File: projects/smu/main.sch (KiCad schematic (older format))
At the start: 2 parts, among them P101 CONN_01X15, P102 CONN_01X34

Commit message: generate net and parts
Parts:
- P102: footprint (none) -> Pin_Headers:Pin_Header_Straight_1x34
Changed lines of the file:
@@
 F 0 "P102" H 5300 4400 50  0000 C CNN
 F 1 "CONN_01X34" V 5400 2650 50  0000 C CNN
-F 2 "" H 5300 2650 50  0000 C CNN
+F 2 "Pin_Headers:Pin_Header_Straight_1x34" H 5300 2650 50  0001 C CNN
 F 3 "" H 5300 2650 50  0000 C CNN
 	1    5300 2650

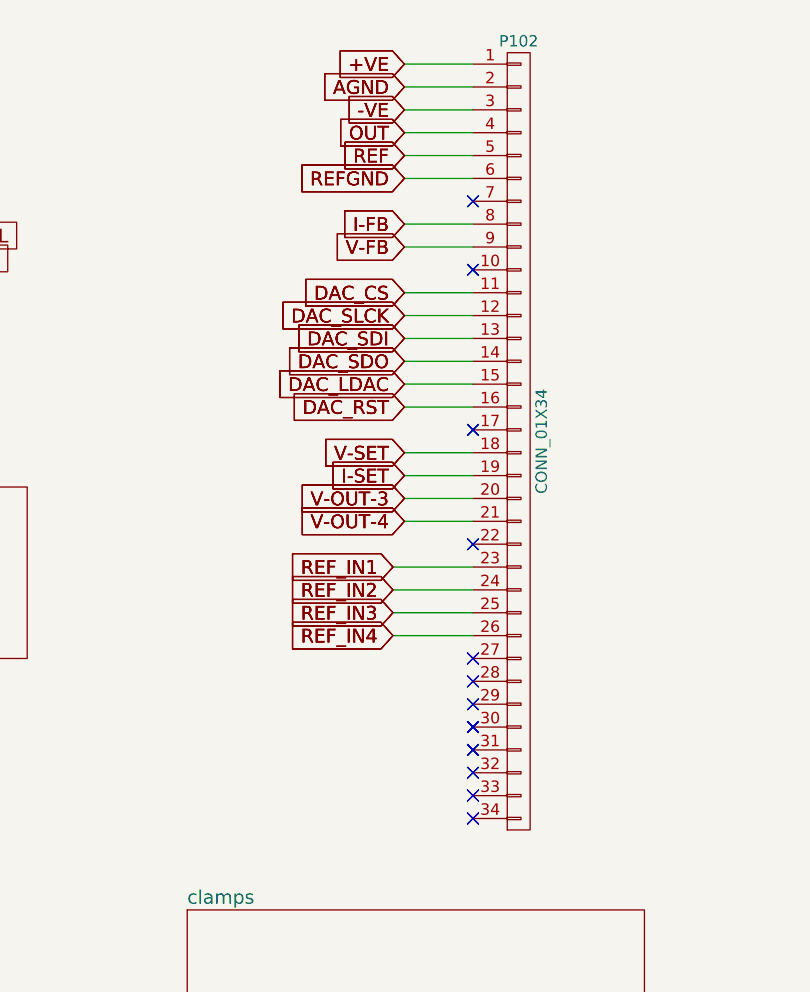
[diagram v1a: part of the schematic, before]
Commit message: do edges again
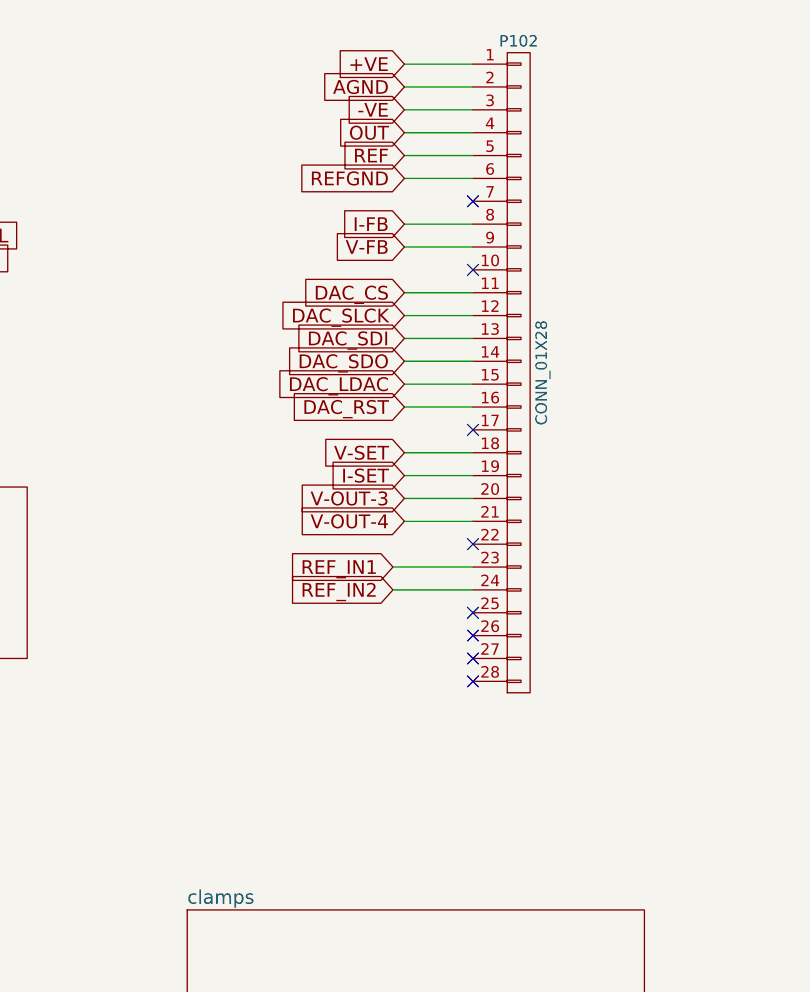
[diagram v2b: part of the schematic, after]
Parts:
- removed P102: CONN_01X34, Pin_Headers:Pin_Header_Straight_1x34, symbol CONN_01X34
- added P102: CONN_01X28, Pin_Headers:Pin_Header_Straight_1x28, symbol CONN_01X28
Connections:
- net +VE: now also P102.1 (P1)
- net -VE: now also P102.3 (P3)
- net AGND: now also P102.2 (P2), P102.6 (P6)
- net DAC_CS: now also P102.11 (P11)
- net DAC_LDAC: now also P102.15 (P15)
- net DAC_RST: now also P102.16 (P16)
- net DAC_SDI: now also P102.13 (P13)
- net DAC_SDO: now also P102.14 (P14)
- net DAC_SLCK: now also P102.12 (P12)
- net I-FB: now also P102.8 (P8)
- net I-SET: now also P102.19 (P19)
- net OUT: now also P102.4 (P4)
- net REF: now also P102.5 (P5)
- net REF_IN1: now also P102.23 (P23)
- net REF_IN2: now also P102.24 (P24)
- net V-FB: now also P102.9 (P9)
- net V-OUT-3: now also P102.20 (P20)
- net V-OUT-4: now also P102.21 (P21)
- net V-SET: now also P102.18 (P18)
- no-connect marks 24 -> 8
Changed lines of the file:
@@
 Wire Wire Line
 	2400 2350 2150 2350
-Text GLabel 4800 1000 0    60   Input ~ 0
-+VE
-Text GLabel 4800 1200 0    60   Input ~ 0
--VE
-Text GLabel 4800 1100 0    60   Input ~ 0
-AGND
-Text GLabel 4800 1400 0    60   Input ~ 0
-REF
 Wire Wire Line
 	5100 1000 4800 1000
@@
 Wire Wire Line
 	5100 1300 4800 1300
-Text GLabel 4800 1700 0    60   Input ~ 0
-I-FB
-Text GLabel 4800 1300 0    60   Input ~ 0
-OUT
-NoConn ~ 5100 1900
-Text GLabel 4800 1800 0    60   Input ~ 0
-V-FB
 Wire Wire Line
 	4800 1400 5100 1400
@@
 Wire Wire Line
 	7650 1300 7650 1500
-Text GLabel 4800 2900 0    60   Input ~ 0
-V-OUT-3
-Text GLabel 4800 3000 0    60   Input ~ 0
-V-OUT-4
-Text GLabel 4800 2000 0    60   Input ~ 0
-DAC_CS
-Text GLabel 4800 2100 0    60   Input ~ 0
-DAC_SLCK
-Text GLabel 4800 2200 0    60   Input ~ 0
-DAC_SDI
-Text GLabel 4800 2300 0    60   Input ~ 0
-DAC_SDO
-Text GLabel 4800 2400 0    60   Input ~ 0
-DAC_LDAC
-Text GLabel 4800 2500 0    60   Input ~ 0
-DAC_RST
 Wire Wire Line
 	4800 2000 5100 2000
@@
 Wire Wire Line
 	4800 2800 5100 2800
-Text GLabel 4800 2700 0    60   Input ~ 0
-V-SET
-Text GLabel 4800 2800 0    60   Input ~ 0
-I-SET
 Wire Wire Line
 	4800 2900 5100 2900
 Wire Wire Line
 	4800 3000 5100 3000
-NoConn ~ 5100 1600
-NoConn ~ 5100 2600
-Text GLabel 4750 3200 0    60   Input ~ 0
-REF_IN1
-Text GLabel 4750 3300 0    60   Input ~ 0
-REF_IN2
-Text GLabel 4750 3400 0    60   Input ~ 0
-REF_IN3
-Text GLabel 4750 3500 0    60   Input ~ 0
-REF_IN4
 Wire Wire Line
 	4750 3200 5100 3200
 Wire Wire Line
 	4750 3300 5100 3300
-Wire Wire Line
-	4750 3400 5100 3400
-Wire Wire Line
-	4750 3500 5100 3500
-NoConn ~ 5100 3100
-NoConn ~ 5100 3600
-NoConn ~ 5100 3700
-NoConn ~ 5100 3800
-NoConn ~ 5100 3900
-NoConn ~ 5100 4000
-NoConn ~ 5100 4100
-NoConn ~ 5100 4200
-NoConn ~ 5100 4300
-Text GLabel 4800 1500 0    60   Input ~ 0
-REFGND
 Wire Wire Line
 	4800 1500 5100 1500
@@
 NoConn ~ 5100 1600
 NoConn ~ 5100 2600
-$Comp
-L CONN_01X34 P102
-U 1 1 58A9E4F4
-P 5300 2650
-F 0 "P102" H 5300 4400 50  0000 C CNN
-F 1 "CONN_01X34" V 5400 2650 50  0000 C CNN
-F 2 "Pin_Headers:Pin_Header_Straight_1x34" H 5300 2650 50  0001 C CNN
-F 3 "" H 5300 2650 50  0000 C CNN
-	1    5300 2650
-	1    0    0    -1
-$EndComp
-Text GLabel 4750 3200 0    60   Input ~ 0
-REF_IN1
-Text GLabel 4750 3300 0    60   Input ~ 0
-REF_IN2
-Text GLabel 4750 3400 0    60   Input ~ 0
-REF_IN3
-Text GLabel 4750 3500 0    60   Input ~ 0
-REF_IN4
 NoConn ~ 5100 3100
 NoConn ~ 5100 3600
 NoConn ~ 5100 3700
-NoConn ~ 5100 3800
-NoConn ~ 5100 3900
-NoConn ~ 5100 4000
-NoConn ~ 5100 4100
-NoConn ~ 5100 4200
-NoConn ~ 5100 4300
 Text GLabel 4800 1500 0    60   Input ~ 0
 REFGND
+$Comp
+L CONN_01X28 P102
+U 1 1 58A96BF2
+P 5300 2350
+F 0 "P102" H 5300 3800 50  0000 C CNN
+F 1 "CONN_01X28" V 5400 2350 50  0000 C CNN
+F 2 "Pin_Headers:Pin_Header_Straight_1x28" H 5300 2350 50  0001 C CNN
+F 3 "" H 5300 2350 50  0000 C CNN
+	1    5300 2350
+	1    0    0    -1
+$EndComp
+Text GLabel 4750 3300 0    60   Input ~ 0
+REF_IN2
+Text GLabel 4750 3200 0    60   Input ~ 0
+REF_IN1
+NoConn ~ 5100 3400
+NoConn ~ 5100 3500
 $EndSCHEMATC
